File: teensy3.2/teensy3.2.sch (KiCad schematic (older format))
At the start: 30 parts

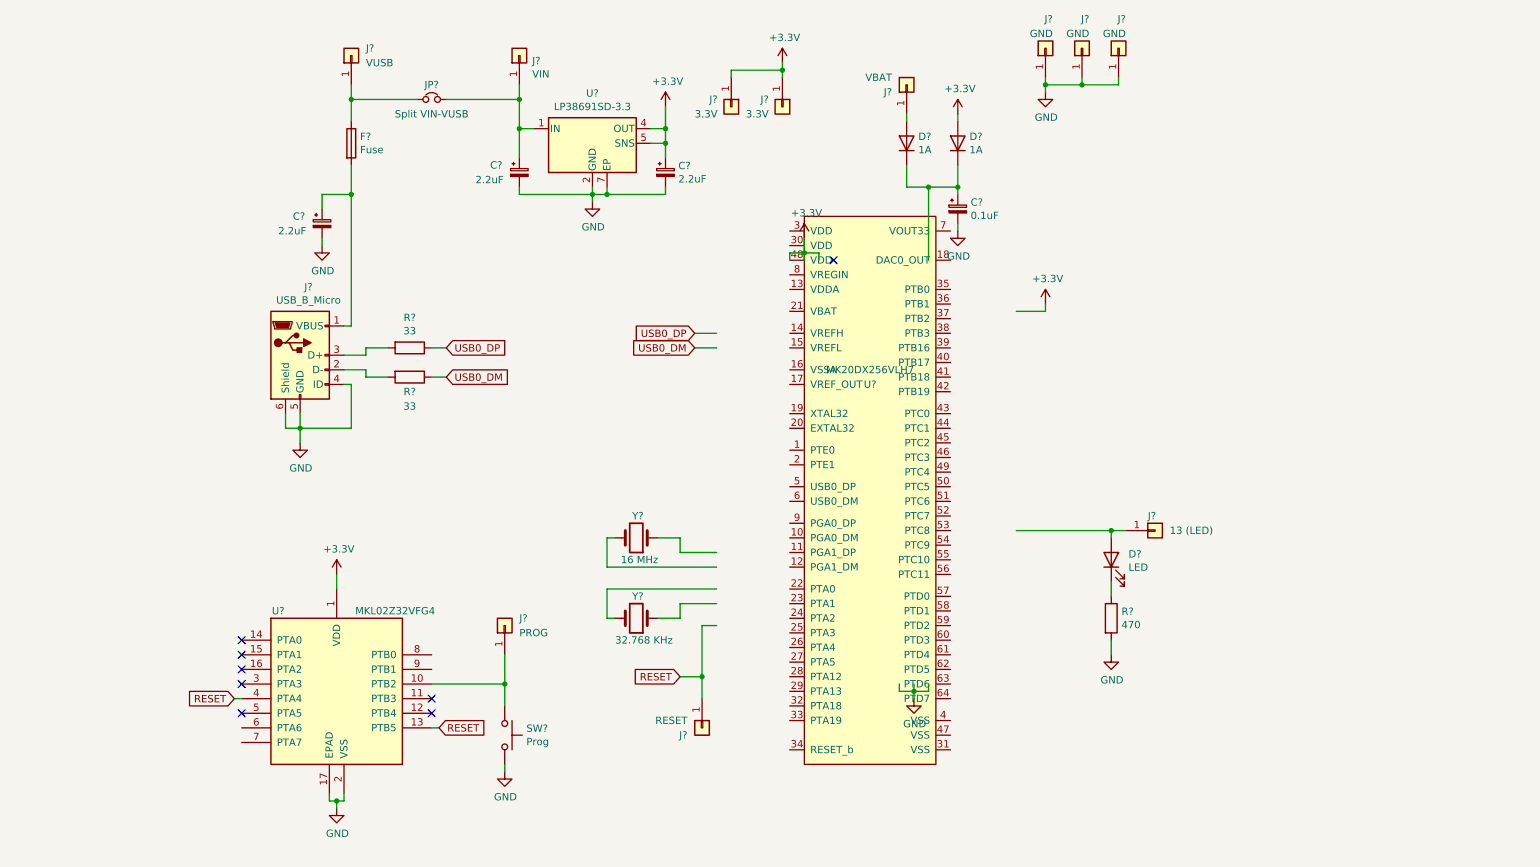
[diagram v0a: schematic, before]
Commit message: ERC ok
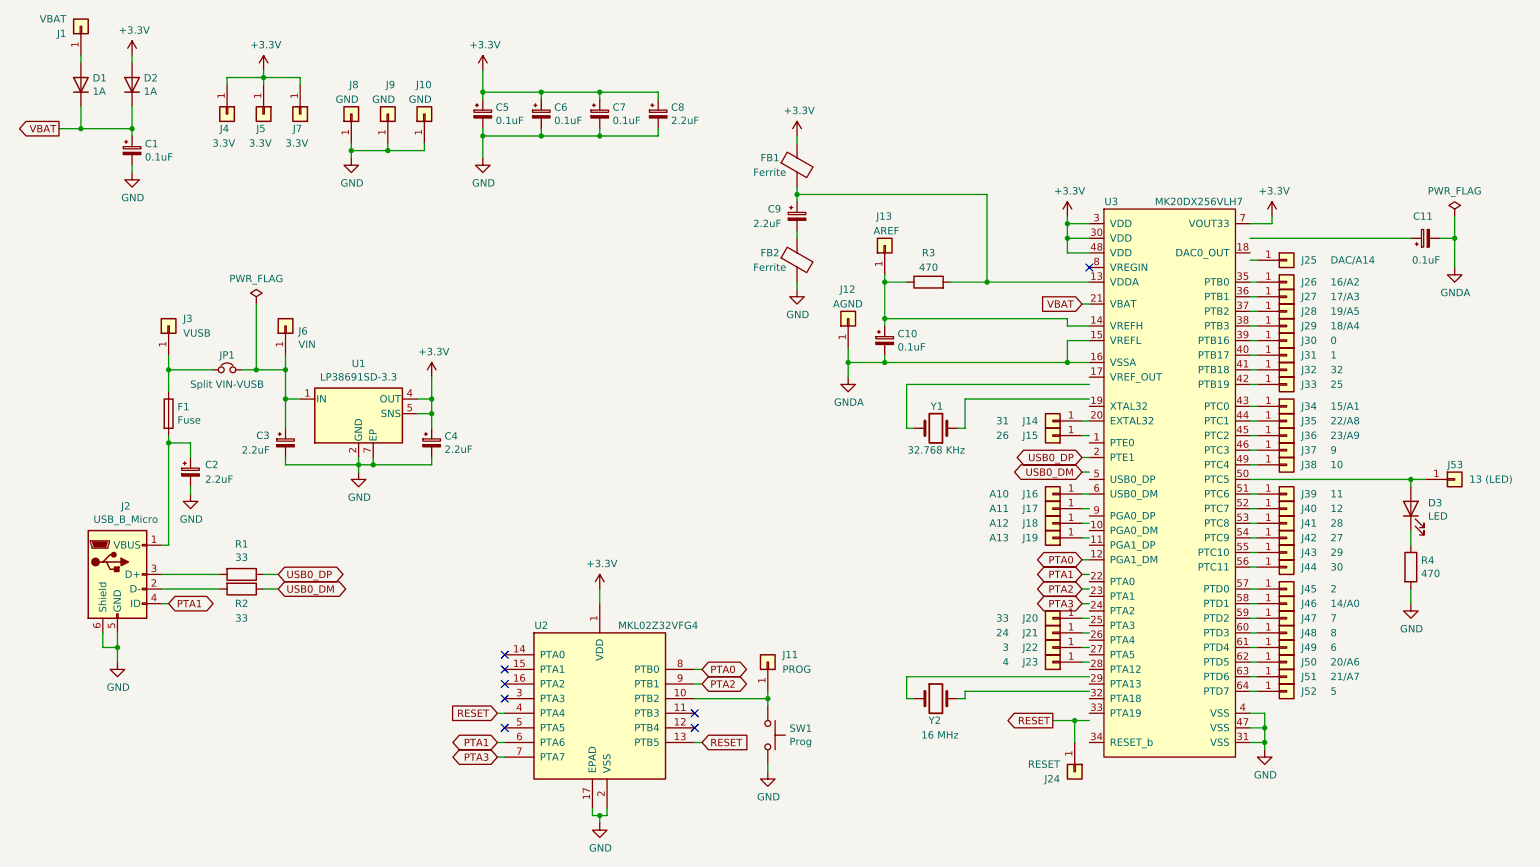
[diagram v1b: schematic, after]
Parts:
- removed Y?: 16 MHz, symbol Device:Crystal
- added C10, C11, C5, C6, C7: 0.1uF, symbol Device:CP_Small
- added C8, C9: 2.2uF, symbol Device:CP_Small
- added FB1, FB2: Ferrite, symbol Device:Ferrite_Bead
- added J12: AGND, TestPoint:TestPoint_Bridge_Pitch2.0mm_Drill0.7mm, symbol Connector_Generic:Conn_01x01
- added J13: AREF, TestPoint:TestPoint_Bridge_Pitch2.0mm_Drill0.7mm, symbol Connector_Generic:Conn_01x01
- added J14: 31, TestPoint:TestPoint_Bridge_Pitch2.0mm_Drill0.7mm, symbol Connector_Generic:Conn_01x01
- added J15: 26, TestPoint:TestPoint_Bridge_Pitch2.0mm_Drill0.7mm, symbol Connector_Generic:Conn_01x01
- added J16: A10, TestPoint:TestPoint_Bridge_Pitch2.0mm_Drill0.7mm, symbol Connector_Generic:Conn_01x01
- added J17: A11, TestPoint:TestPoint_Bridge_Pitch2.0mm_Drill0.7mm, symbol Connector_Generic:Conn_01x01
- added J18: A12, TestPoint:TestPoint_Bridge_Pitch2.0mm_Drill0.7mm, symbol Connector_Generic:Conn_01x01
- added J19: A13, TestPoint:TestPoint_Bridge_Pitch2.0mm_Drill0.7mm, symbol Connector_Generic:Conn_01x01
- added J20: 33, TestPoint:TestPoint_Bridge_Pitch2.0mm_Drill0.7mm, symbol Connector_Generic:Conn_01x01
- added J21: 24, TestPoint:TestPoint_Bridge_Pitch2.0mm_Drill0.7mm, symbol Connector_Generic:Conn_01x01
- added J22: 3, TestPoint:TestPoint_Bridge_Pitch2.0mm_Drill0.7mm, symbol Connector_Generic:Conn_01x01
- added J23: 4, TestPoint:TestPoint_Bridge_Pitch2.0mm_Drill0.7mm, symbol Connector_Generic:Conn_01x01
- added J25: DAC/A14, TestPoint:TestPoint_Bridge_Pitch2.0mm_Drill0.7mm, symbol Connector_Generic:Conn_01x01
- added J26: 16/A2, TestPoint:TestPoint_Bridge_Pitch2.0mm_Drill0.7mm, symbol Connector_Generic:Conn_01x01
- added J27: 17/A3, TestPoint:TestPoint_Bridge_Pitch2.0mm_Drill0.7mm, symbol Connector_Generic:Conn_01x01
- added J28: 19/A5, TestPoint:TestPoint_Bridge_Pitch2.0mm_Drill0.7mm, symbol Connector_Generic:Conn_01x01
- added J29: 18/A4, TestPoint:TestPoint_Bridge_Pitch2.0mm_Drill0.7mm, symbol Connector_Generic:Conn_01x01
- added J30: 0, TestPoint:TestPoint_Bridge_Pitch2.0mm_Drill0.7mm, symbol Connector_Generic:Conn_01x01
- added J31: 1, TestPoint:TestPoint_Bridge_Pitch2.0mm_Drill0.7mm, symbol Connector_Generic:Conn_01x01
- added J32: 32, TestPoint:TestPoint_Bridge_Pitch2.0mm_Drill0.7mm, symbol Connector_Generic:Conn_01x01
- added J33: 25, TestPoint:TestPoint_Bridge_Pitch2.0mm_Drill0.7mm, symbol Connector_Generic:Conn_01x01
- added J34: 15/A1, TestPoint:TestPoint_Bridge_Pitch2.0mm_Drill0.7mm, symbol Connector_Generic:Conn_01x01
- added J35: 22/A8, TestPoint:TestPoint_Bridge_Pitch2.0mm_Drill0.7mm, symbol Connector_Generic:Conn_01x01
- added J36: 23/A9, TestPoint:TestPoint_Bridge_Pitch2.0mm_Drill0.7mm, symbol Connector_Generic:Conn_01x01
- added J37: 9, TestPoint:TestPoint_Bridge_Pitch2.0mm_Drill0.7mm, symbol Connector_Generic:Conn_01x01
- added J38: 10, TestPoint:TestPoint_Bridge_Pitch2.0mm_Drill0.7mm, symbol Connector_Generic:Conn_01x01
- added J39: 11, TestPoint:TestPoint_Bridge_Pitch2.0mm_Drill0.7mm, symbol Connector_Generic:Conn_01x01
- added J40: 12, TestPoint:TestPoint_Bridge_Pitch2.0mm_Drill0.7mm, symbol Connector_Generic:Conn_01x01
- added J41: 28, TestPoint:TestPoint_Bridge_Pitch2.0mm_Drill0.7mm, symbol Connector_Generic:Conn_01x01
- added J42: 27, TestPoint:TestPoint_Bridge_Pitch2.0mm_Drill0.7mm, symbol Connector_Generic:Conn_01x01
- added J43: 29, TestPoint:TestPoint_Bridge_Pitch2.0mm_Drill0.7mm, symbol Connector_Generic:Conn_01x01
- added J44: 30, TestPoint:TestPoint_Bridge_Pitch2.0mm_Drill0.7mm, symbol Connector_Generic:Conn_01x01
- added J45: 2, TestPoint:TestPoint_Bridge_Pitch2.0mm_Drill0.7mm, symbol Connector_Generic:Conn_01x01
- added J46: 14/A0, TestPoint:TestPoint_Bridge_Pitch2.0mm_Drill0.7mm, symbol Connector_Generic:Conn_01x01
- added J47: 7, TestPoint:TestPoint_Bridge_Pitch2.0mm_Drill0.7mm, symbol Connector_Generic:Conn_01x01
- added J48: 8, TestPoint:TestPoint_Bridge_Pitch2.0mm_Drill0.7mm, symbol Connector_Generic:Conn_01x01
- added J49: 6, TestPoint:TestPoint_Bridge_Pitch2.0mm_Drill0.7mm, symbol Connector_Generic:Conn_01x01
- added J50: 20/A6, TestPoint:TestPoint_Bridge_Pitch2.0mm_Drill0.7mm, symbol Connector_Generic:Conn_01x01
- added J51: 21/A7, TestPoint:TestPoint_Bridge_Pitch2.0mm_Drill0.7mm, symbol Connector_Generic:Conn_01x01
- added J52: 5, TestPoint:TestPoint_Bridge_Pitch2.0mm_Drill0.7mm, symbol Connector_Generic:Conn_01x01
- added J7: 3.3V, TestPoint:TestPoint_Bridge_Pitch2.0mm_Drill0.7mm, symbol Connector_Generic:Conn_01x01
- added R3: 470, symbol Device:R
- added Y2: 16 MHz, symbol Device:Crystal
- gave numbers to parts that had none: 29
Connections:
- net labels added: GNDA, PTA0, PTA1, PTA2, PTA3, VBAT
- wire segments 110 -> 197
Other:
- moved on the sheet: C1, C2, C3, C4, D1, D2, D3, F1, J1, J10, J11, J2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
